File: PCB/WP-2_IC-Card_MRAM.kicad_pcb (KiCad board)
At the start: 2 copper layers, 54 x 54 mm, 38 parts, among them J1 SMS-138-01-G-S, SW1 CUS-14TB, U1 MRxA08xxYSxxx, U2 MIC5317-3.3YD5, U3 4245, U4 4245, U5 4245, U6 4245

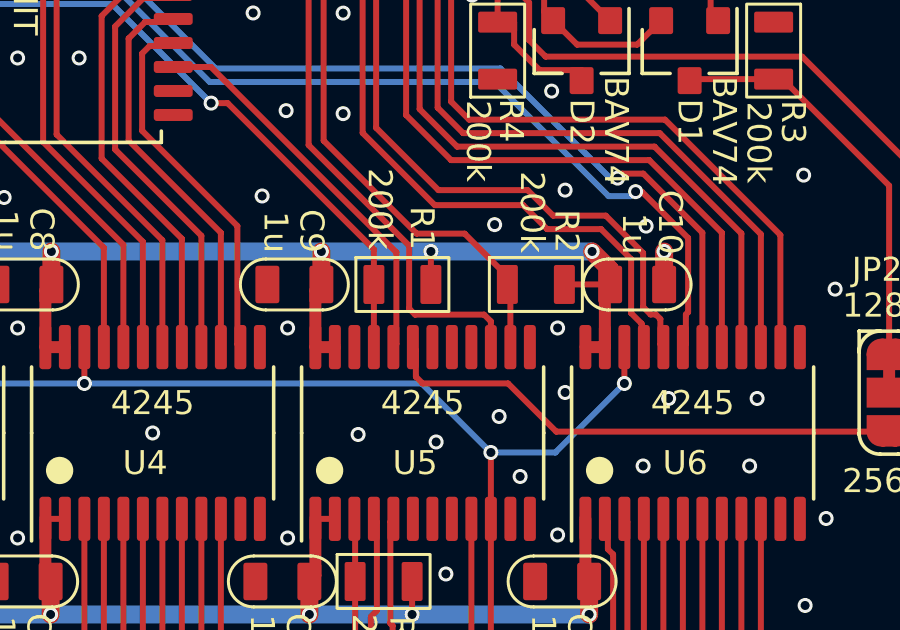
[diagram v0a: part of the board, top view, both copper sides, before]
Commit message: pics
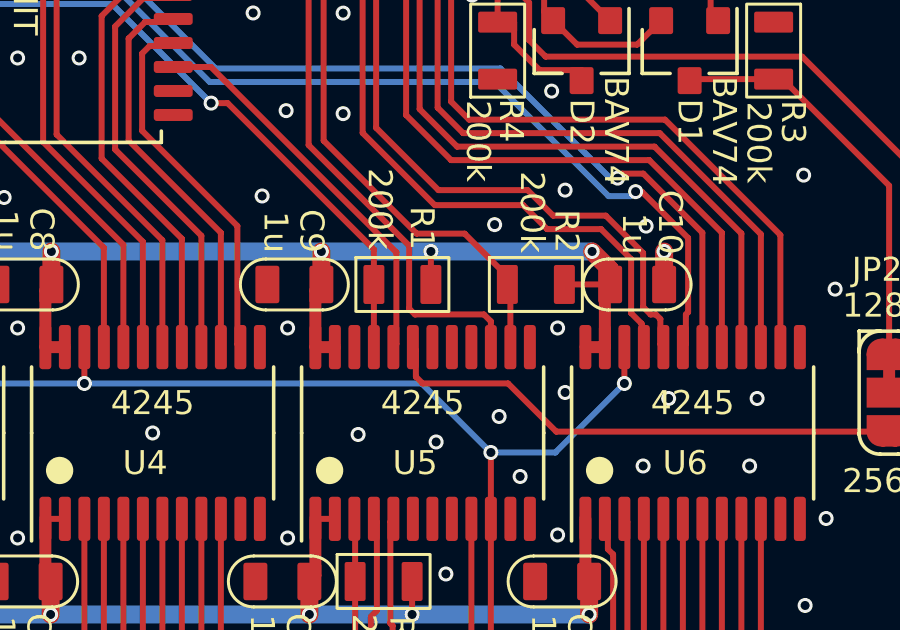
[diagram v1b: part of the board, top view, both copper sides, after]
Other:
- board text added: "3MM ADHESIVE TRANSFER TAPE"
- board text removed: "5 x ADHESIVE TRANSFER 3MM x 42MM"
